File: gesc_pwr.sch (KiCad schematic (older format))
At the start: 45 parts, among them J10 PHASE_C, J11 PHASE_B, J12 NTC, J9 PHASE_A, Q1 TPH2R608NH,L1Q, Q2 TPH2R608NH,L1Q, Q3 TPH2R608NH,L1Q, Q4 TPH2R608NH,L1Q, Q5 TPH2R608NH,L1Q, Q6 TPH2R608NH,L1Q, U4 INA240A2, U5 INA240A2, U6 INA240A2, U7 SN74LVC1G66DBVR, U8 SN74LVC1G66DBVR, U9 SN74LVC1G66DBVR

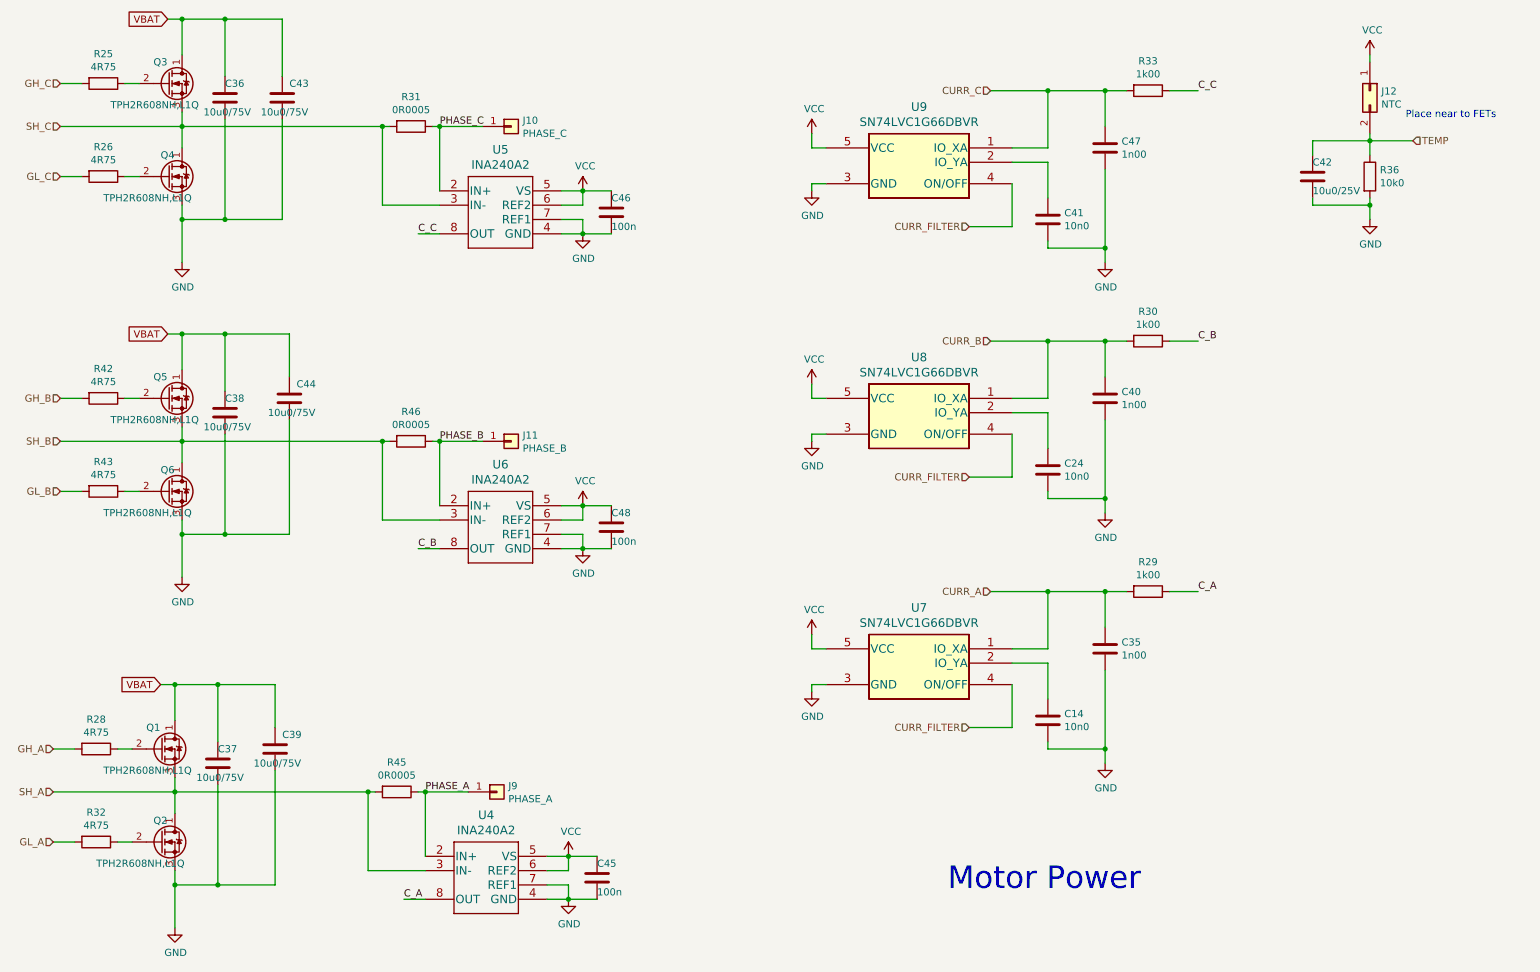
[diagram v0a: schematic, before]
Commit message: save
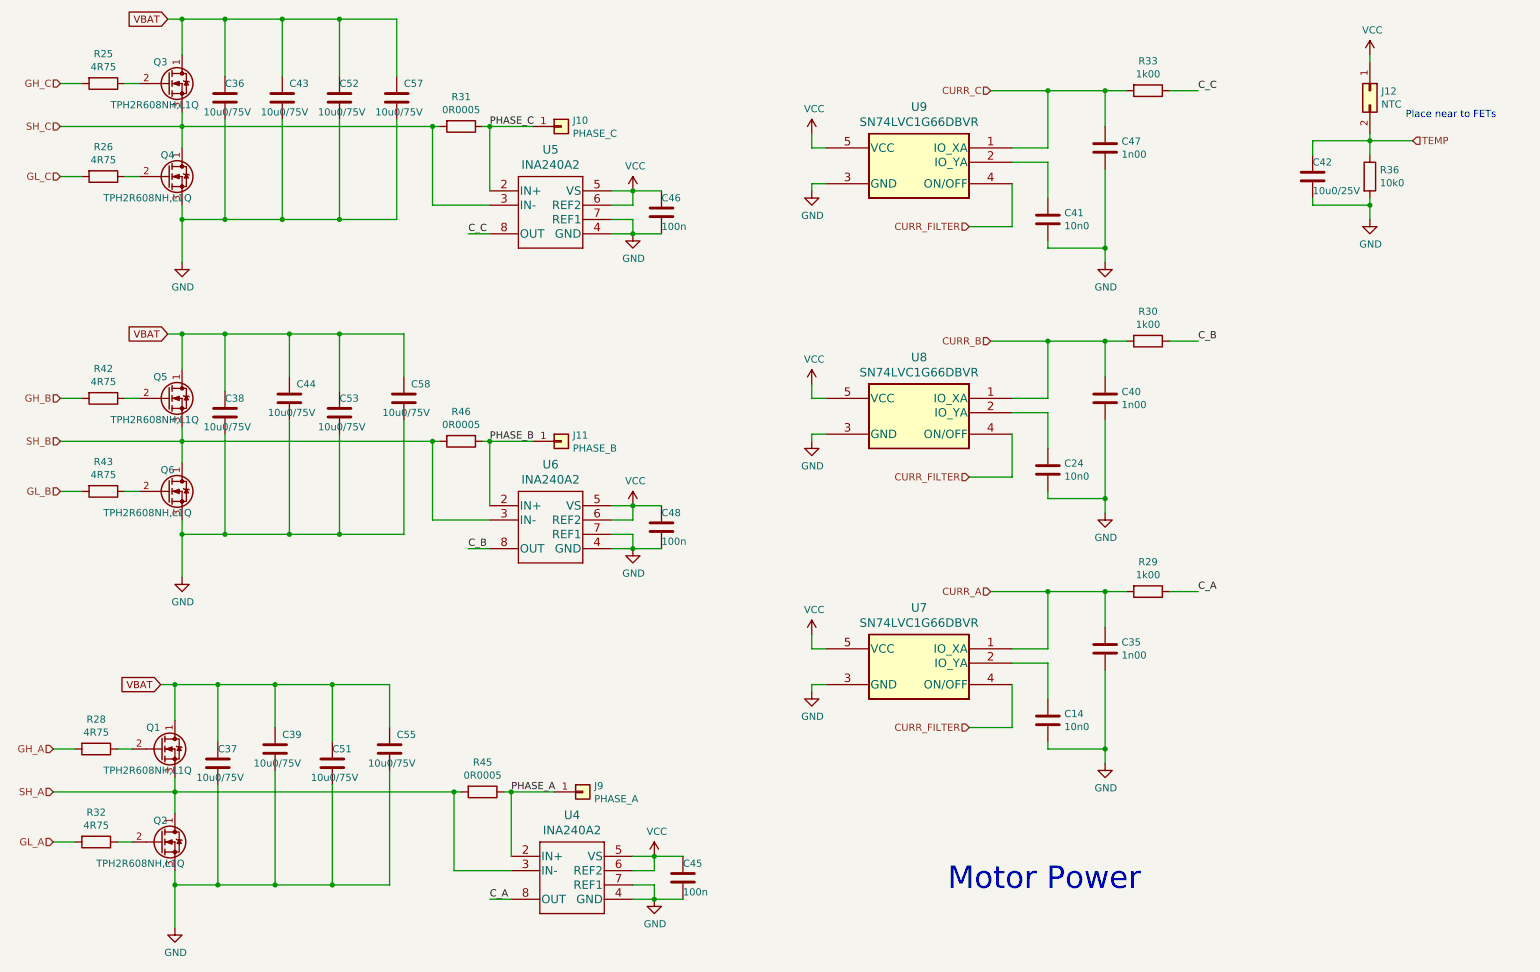
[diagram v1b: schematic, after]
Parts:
- added C51, C52, C53, C55, C57, C58: 10u0/75V, Capacitor_SMD:C_1210_3225Metric, symbol Device:C
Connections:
- net GND: now also C51.2, C52.2, C53.2, C55.2, C57.2, C58.2
- net VBAT: now also C51.1, C52.1, C53.1, C55.1, C57.1, C58.1
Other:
- moved on the sheet: C45, C46, C48, J10, J11, J9, R31, R45, R46, U4, U5, U6
